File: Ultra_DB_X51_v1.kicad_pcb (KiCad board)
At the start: 2 copper layers, 178 x 145 mm, 144 parts, among them IC1 L293D, J1 USB_2, K1 RELAYPTH, K2 RELAYPTH, K3 I2C, K4 CONN_3, P1 CONN_5, P10 CONN_8, P11 CONN_4, P12 CONN_8, P13 CONN_1, P14 CONN_1, P15 CONN_1, P16 CONN_8, P17 CONN_8, P18 CONN_7, P19 CONN_1, P2 CONN_5, P3 CONN_5, P4 CONN_1, P5 CONN_5X2, P6 CONN_1, P7 CONN_8, P8 CONN_8, P9 CONN_8, Q1 BC557, Q2 BC548, Q3 BC548, Q4 BC548, Q5 BC548, Q6 BC548, Q7 BC548, Q8 BC548, SW1 SPST, SW10 5, SW11 6, SW12 7, SW13 8, SW14 1, SW15 2, SW16 3, SW17 4, SW18 SPST, SW19 INT0, SW2 C, SW20 INT1, SW3 D, SW4 E, SW5 F, SW6 9, SW7 0, SW8 A, SW9 B, U1 7805, U10 CP2102, U2 24C16, U3 DS1307, U4 BATTERY, U5 LM555N_XL, U6 ADC0808, U7 AT89S52, X1 CRYSTAL, X3 11.0592MHz

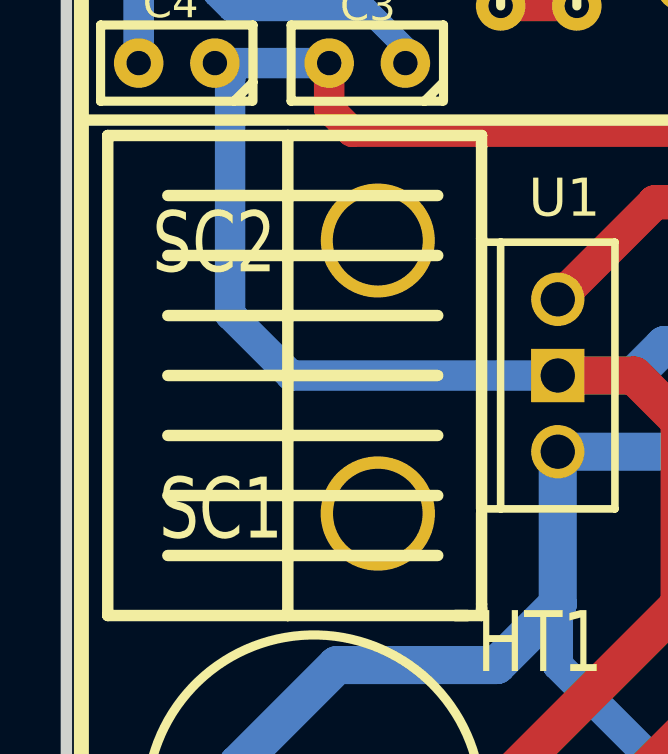
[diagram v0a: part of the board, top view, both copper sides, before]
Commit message: Gerber file generated
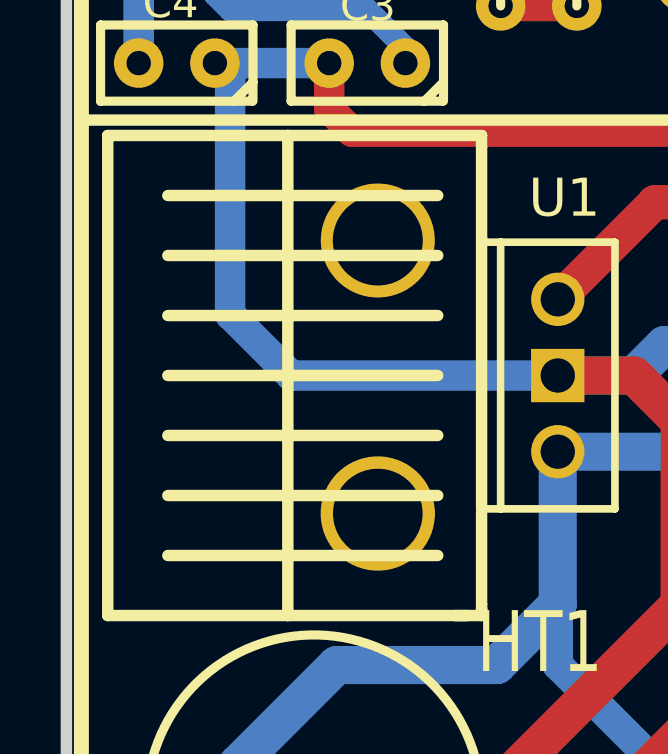
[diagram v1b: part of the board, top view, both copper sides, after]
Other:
- board text removed: "SC1"
- board text removed: "SC2"
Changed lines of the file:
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@@
-(kicad_pcb (version 4) (host pcbnew "(2015-01-16 BZR 5376)-product")
+(kicad_pcb (version 4) (host pcbnew 4.0.4-stable)
   (general
     (links 402)
     (no_connects 0)
-    (area 59.187362 29.286818 245.192772 175.577)
+    (area 59.286818 29.286818 237.690501 175.7294)
     (thickness 1.6002)
-    (drawings 172)
+    (drawings 170)
     (tracks 1489)
     (zones 0)
@@
   )
   (layers
-    (0 Front signal hide)
-    (31 Back signal hide)
+    (0 Front signal)
+    (31 Back signal)
     (32 B.Adhes user)
     (33 F.Adhes user)
@@
     (mod_text_size 1.524 1.524)
     (mod_text_width 0.3048)
-    (pad_size 3.81 3.81)
-    (pad_drill 2.9845)
+    (pad_size 4.064 4.064)
+    (pad_drill 3.048)
     (pad_to_mask_clearance 0.254)
     (aux_axis_origin 0 0)
@@
     )
     (fp_circle (center 0 0) (end 0 -2.286) (layer F.SilkS) (width 0.381))
-    (pad "" thru_hole circle (at 0 0) (size 4.064 4.064) (drill 3.048) (layers *.Cu *.Mask F.SilkS))
+    (pad "" np_thru_hole circle (at 0 0) (size 4.064 4.064) (drill 3.048) (layers *.Cu *.Mask))
   )
   (module 1pin (layer Front)
@@
     )
     (fp_circle (center 0 0) (end 0 -2.286) (layer F.SilkS) (width 0.381))
-    (pad "" thru_hole circle (at 0 0) (size 4.064 4.064) (drill 3.048) (layers *.Cu *.Mask F.SilkS))
+    (pad "" np_thru_hole circle (at 0 0) (size 4.064 4.064) (drill 3.048) (layers *.Cu *.Mask))
   )
   (module 1pin (layer Front)
@@
     )
     (fp_circle (center 0 0) (end 0 -2.286) (layer F.SilkS) (width 0.381))
-    (pad "" thru_hole circle (at 0 0) (size 4.064 4.064) (drill 3.048) (layers *.Cu *.Mask F.SilkS))
+    (pad "" np_thru_hole circle (at 0 0) (size 4.064 4.064) (drill 3.048) (layers *.Cu *.Mask))
   )
   (module HC-49V (layer Front)
@@
     )
     (fp_circle (center 0 0) (end 0 -2.286) (layer F.SilkS) (width 0.381))
-    (pad "" thru_hole circle (at 0 0) (size 4.064 4.064) (drill 3.048) (layers *.Cu *.Mask F.SilkS))
+    (pad "" np_thru_hole circle (at 0 0) (size 4.064 4.064) (drill 3.048) (layers *.Cu *.Mask))
   )
   (module "logo:LOGO (1)" (layer Back)
@@
     )
     (fp_circle (center 0 0) (end 0 -2.286) (layer F.SilkS) (width 0.15))
-    (pad 1 thru_hole circle (at 0 0) (size 4.064 4.064) (drill 3.048) (layers *.Cu *.Mask F.SilkS))
+    (pad "" np_thru_hole circle (at 0 0) (size 4.064 4.064) (drill 3.048) (layers *.Cu *.Mask))
   )
   (module Connect:1pin (layer Front)
@@
     )
     (fp_circle (center 0 0) (end 0 -2.286) (layer F.SilkS) (width 0.15))
-    (pad 1 thru_hole circle (at 0 0) (size 4.064 4.064) (drill 3.048) (layers *.Cu *.Mask F.SilkS))
+    (pad "" np_thru_hole circle (at 0 0) (size 4.064 4.064) (drill 3.048) (layers *.Cu *.Mask))
   )
   (module Connect:1pin (layer Front)
@@
     )
     (fp_circle (center 0 0) (end 0 -2.286) (layer F.SilkS) (width 0.15))
-    (pad 1 thru_hole circle (at 0 0) (size 4.064 4.064) (drill 3.048) (layers *.Cu *.Mask F.SilkS))
-  )
-  (gr_text SC2 (at 64.425 130.65) (layer F.SilkS)
-    (effects (font (size 2.032 1.524) (thickness 0.3048)))
-  )
-  (gr_text SC1 (at 64.65 139.525) (layer F.SilkS)
-    (effects (font (size 2.032 1.524) (thickness 0.3048)))
+    (pad "" np_thru_hole circle (at 0 0) (size 4.064 4.064) (drill 3.048) (layers *.Cu *.Mask))
   )
   (gr_text HT1 (at 75.275 143.975) (layer F.SilkS)
